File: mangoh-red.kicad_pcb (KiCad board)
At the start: 6 copper layers, 70 x 61.8 mm, 598 parts, among them CN1000 uFL, CN301 uFL, CN302 uFL, CN303 uFL, CN304 USB_A, CN305 USB_B_Micro, CN306 Conn_02x19_Counter_Clockwise, CN307 Conn_02x13_Odd_Even, CN310 Conn_02x03_Odd_Even, CN312 Conn_02x03_Odd_Even, CN400 Conn_02x05_Odd_Even, CN401 Conn_02x05_Odd_Even, CN500 JP036-RT3B4AB, CN600 CN600, CN801 USB_B_Micro, CN802 Conn_01x02, CN804 Conn_01x03, J200 CF3-Socket, Q312 NSBC114YDP6T5G, Q400 NSBC114YDP6T5G, Q405 NSBC114YDP6T5G, Q600 PDTC115EM, SW200 PTS810, SW400 SKTDLDE010, SW401 Conn_02x08_Counter_Clockwise, SW402 SKTDLDE010, U1000 MT7697, U1001 MX25L3233FM1I-08G_TR, U1004 SX1509BIULTRT, U1005 TPS61253YFFR, U1006 CP2130-F01-GM, U1007 24AA32AF-I-MNY, U1010 74LVC2G126HD4-7, U1020 74LVC2G126HD4-7, U301 FT230XQ-R, U302 TS3A5018RSVR, U304 74LVC2G126HD4-7, U306 FXMA108BQX, U307 FXMA108BQX, U337 FXMA108BQX, U400 NCP303LSN30T1G, U401 74AUP1G08GM, U402 74AUP1G08GM, U404 TCA9546APWR, U405 74AUP1G08GM, U500 WM8944BECS_R, U501 TS3A5018RSVR, U600 XC6223H29B9R-G, U603 ESIM, U610 TXS02612ZQSR, U701 USB3503A-1-GL-TR, U702 MIC2026-1YM, U704 BMI160, U705 BMP280, U706 PNJ4K01F, U800 BQ24296RGER, U801 LTC2942IDCB_TRMPBF, U900 TPS7A7300, U901 TPS62420DRC, U903 XC6221A182MR, Y1000 CT2520DB26000C0FZZA1

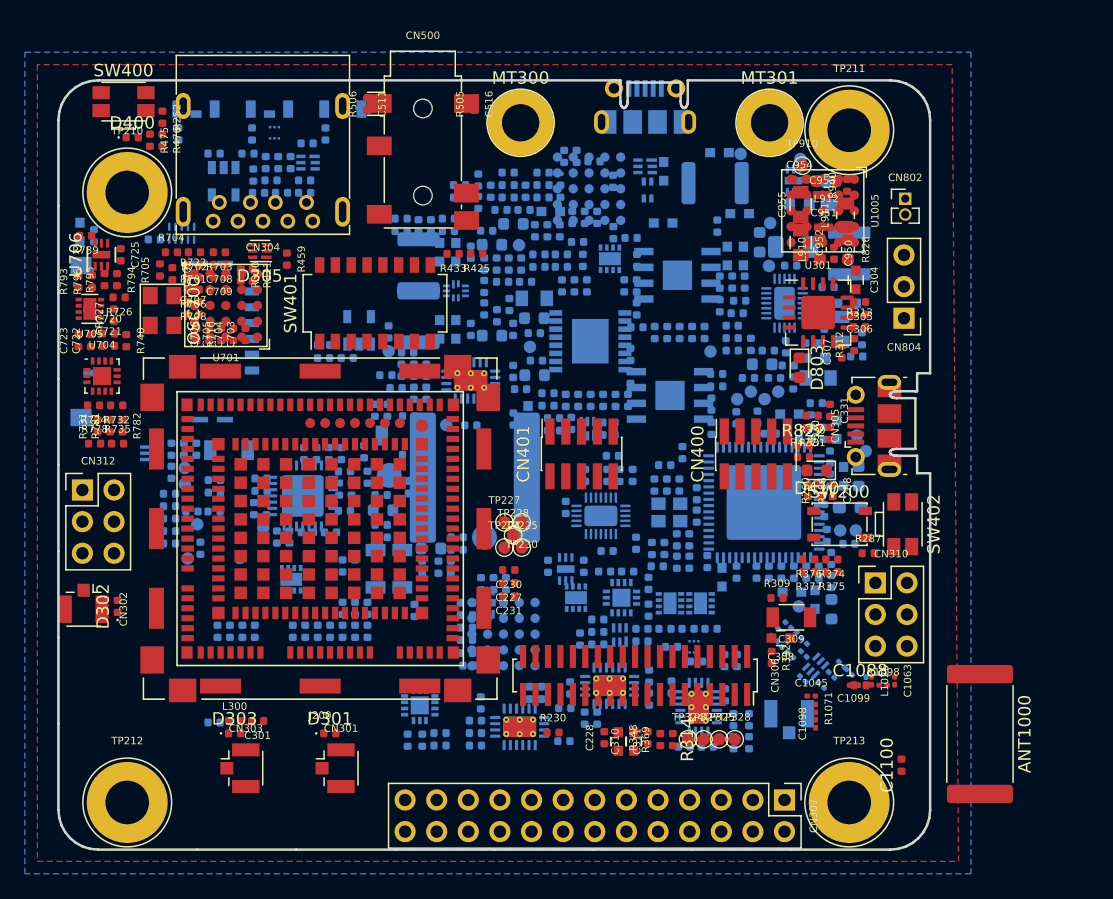
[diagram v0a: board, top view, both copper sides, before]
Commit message: Update
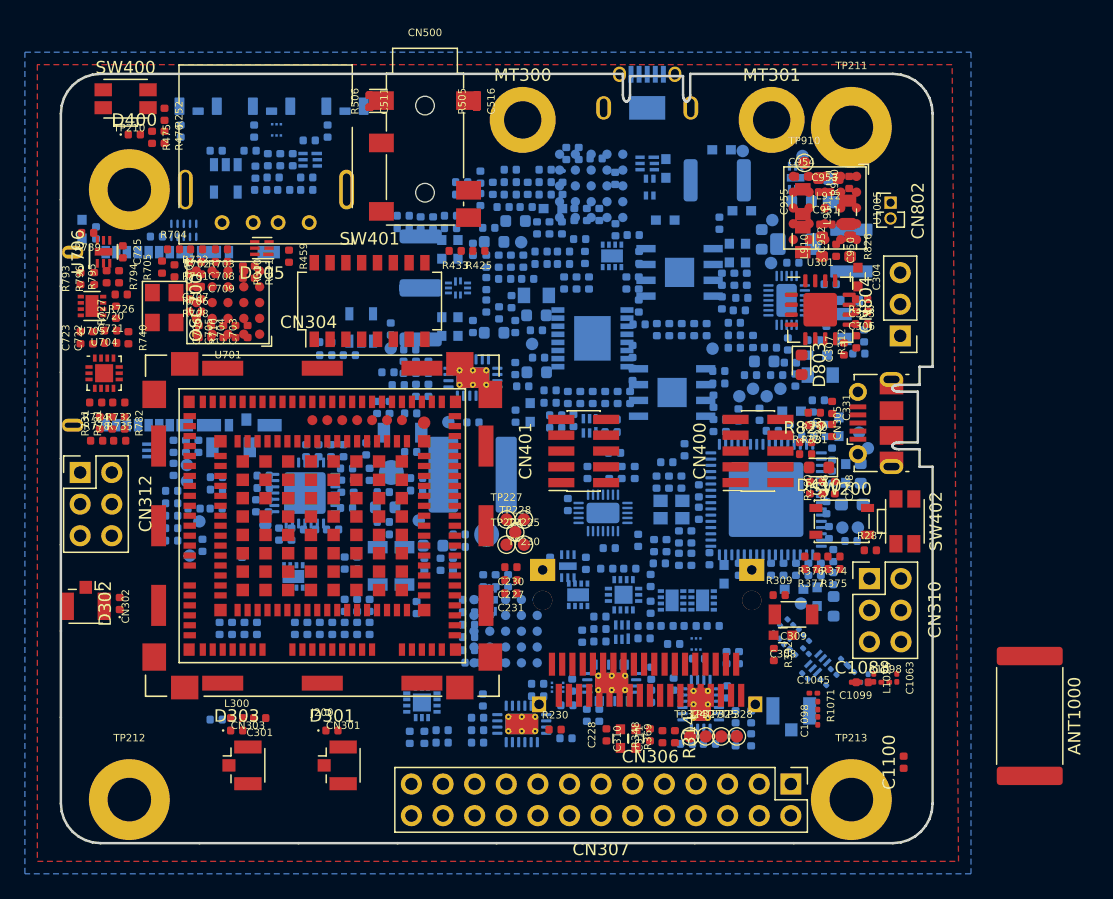
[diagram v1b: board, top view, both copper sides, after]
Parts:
- CN304: footprint Connector_USB:USB3_A_Molex_48393-001 -> MangOH-Red:CONN_4P_1450x1400_USB_2GND_RA_THRU
- CN306: footprint Connector_PinSocket_1.00mm:PinSocket_2x19_P1.00mm_Vertical_SMD -> MangOH-Red:CONN_38P_1820x1150_0080CC_EVERCLEAR
- CN307: footprint Connector_PinHeader_2.54mm:PinHeader_2x13_P2.54mm_Vertical -> MangOH-Red:CONN_26P_3300x0483_0254CC_HEADER_THRU
- CN310, CN312: footprint Connector_PinHeader_2.54mm:PinHeader_2x03_P2.54mm_Vertical -> MangOH-Red:CONN_6P_0760x0510_HEADER_THRU_0254CC
- CN400, CN401: footprint Connector_PinSocket_1.27mm:PinSocket_2x05_P1.27mm_Vertical_SMD -> MangOH-Red:CONN_10P_0673x0305_0127CC_SMT
- CN801: footprint Connector_USB:USB_Micro-B_Molex-105017-0001 -> MangOH-Red:CONN_5P_0750x0560_USB_5GND_HRS_ZX62RD
- CN802: footprint Connector_PinHeader_1.27mm:PinHeader_1x02_P1.27mm_Vertical -> MangOH-Red:CONN_2P_0590x0450_0200CC_THRU_HEADER
- CN804: footprint Connector_PinHeader_2.54mm:PinHeader_1x03_P2.54mm_Vertical -> MangOH-Red:CONN_3P_0762x0254_VERTICAL_HEADER_SINGLE_ROW_THRU_SAMTEC_TSW
- SW401: footprint Button_Switch_SMD:SW_DIP_SPSTx08_Slide_Omron_A6H-8101_W6.15mm_P1.27mm -> MangOH-Red:SW_16P_1128x0620_0127CC_DIP_SPST
- moved CN307 14.7 mm to (163.4, 113.3), turned to 180 degrees
- moved ANT1000 4.25 mm to (197.8, 106.6)
- moved CN310 2.29 mm to (186.2, 98.0), turned to 270 degrees
- moved CN306 1.61 mm to (167.1, 102.0), turned to 180 degrees
- moved CN312 1.53 mm to (122.8, 89.5), turned to 270 degrees
- moved CN802 1.53 mm to (186.7, 66.0), turned to 270 degrees
- moved CN304 1.48 mm to (139.9, 66.8)
- moved CN804 1.12 mm to (187.4, 73.5), turned to 90 degrees
- moved SW401 0.47 mm to (144.8, 73.2), turned to 0 degrees
- moved C1000 0.29 mm to (168.7, 86.2)
- moved C1006 0.29 mm to (177.2, 83.7)
- moved C1015 0.29 mm to (182.1, 93.7)
- moved C1020 0.29 mm to (178.1, 94.8)
- moved C1021 0.29 mm to (169.7, 94.0)
- moved C1024 0.29 mm to (173.3, 95.2)
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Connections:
- J200 pad 27: (no net) -> UIM1_CLK
- J200 pad 29: (no net) -> UIM1_RESET
- R600 pad 2: (no net) -> Net-(CN600-PadT5)
